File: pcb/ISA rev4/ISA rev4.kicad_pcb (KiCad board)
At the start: 2 copper layers, 109 x 51.1 mm, 38 parts, among them J1 PCB_Finger_ISA_8bit, J2 OLED Header, J3 remote header, J4 OLED here, J5 Button Header, SW1 Up, SW2 Down, SW3 Select/Menu, U1 74LVC02, U2 74LVC02, U3 74LVC245, U4 74LVC245, U5 74LVC245, U6 Pico

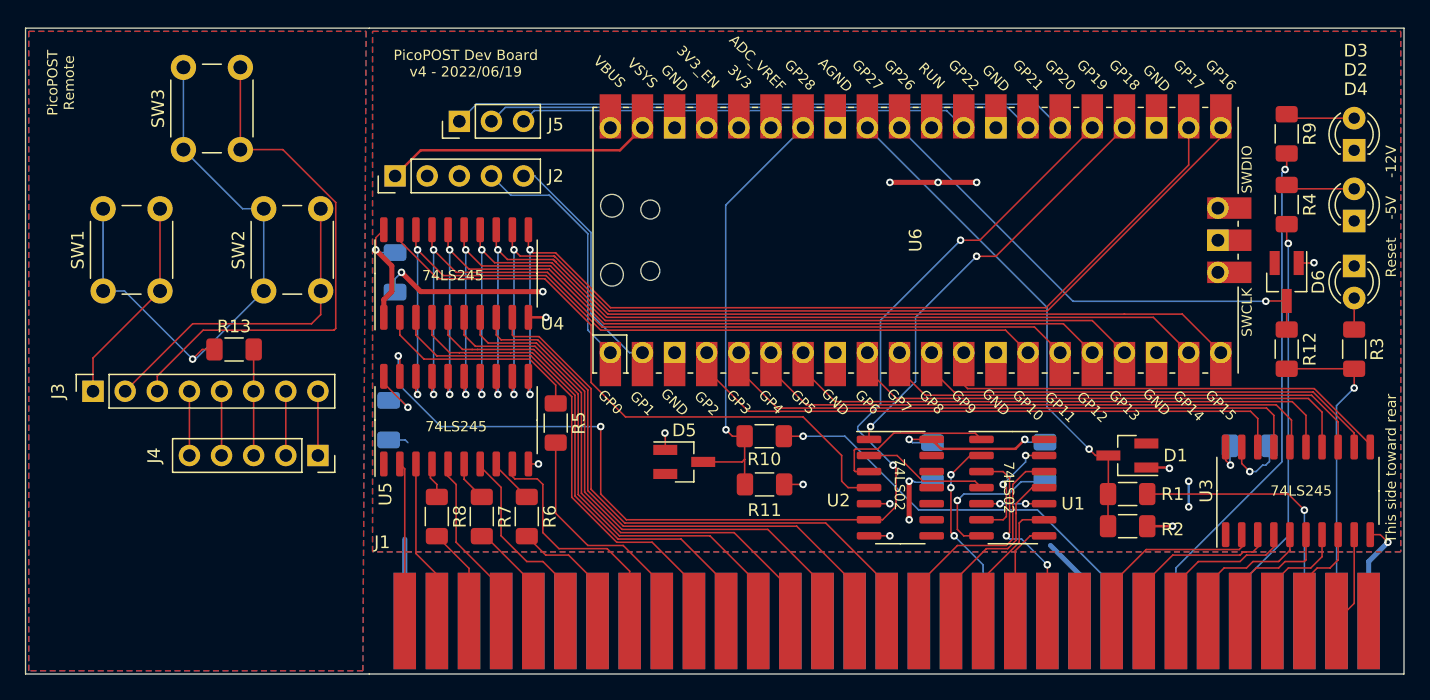
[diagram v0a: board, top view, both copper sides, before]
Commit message: PCB revision 5
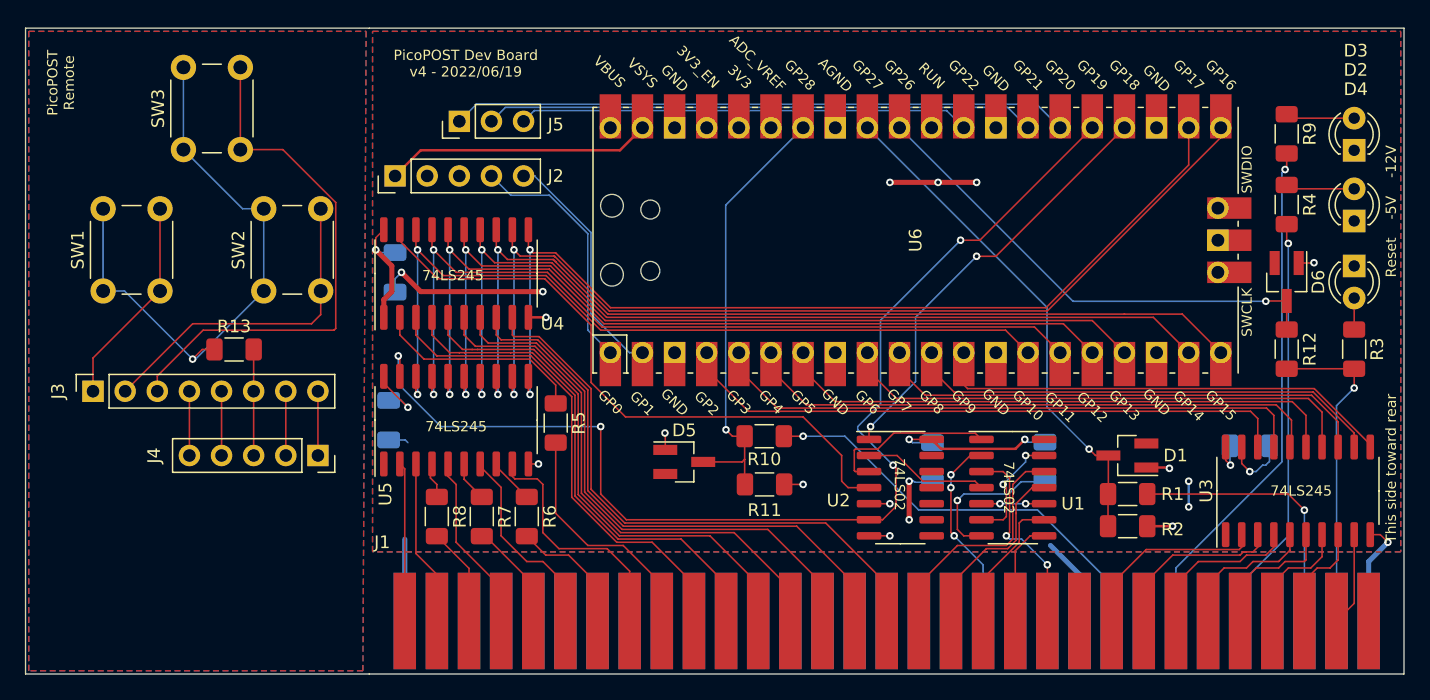
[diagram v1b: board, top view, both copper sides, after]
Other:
- board text added: "V-Cut here"
